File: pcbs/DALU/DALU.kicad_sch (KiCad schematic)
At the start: 1 part, among them J101 Conn_02x20_Odd_Even

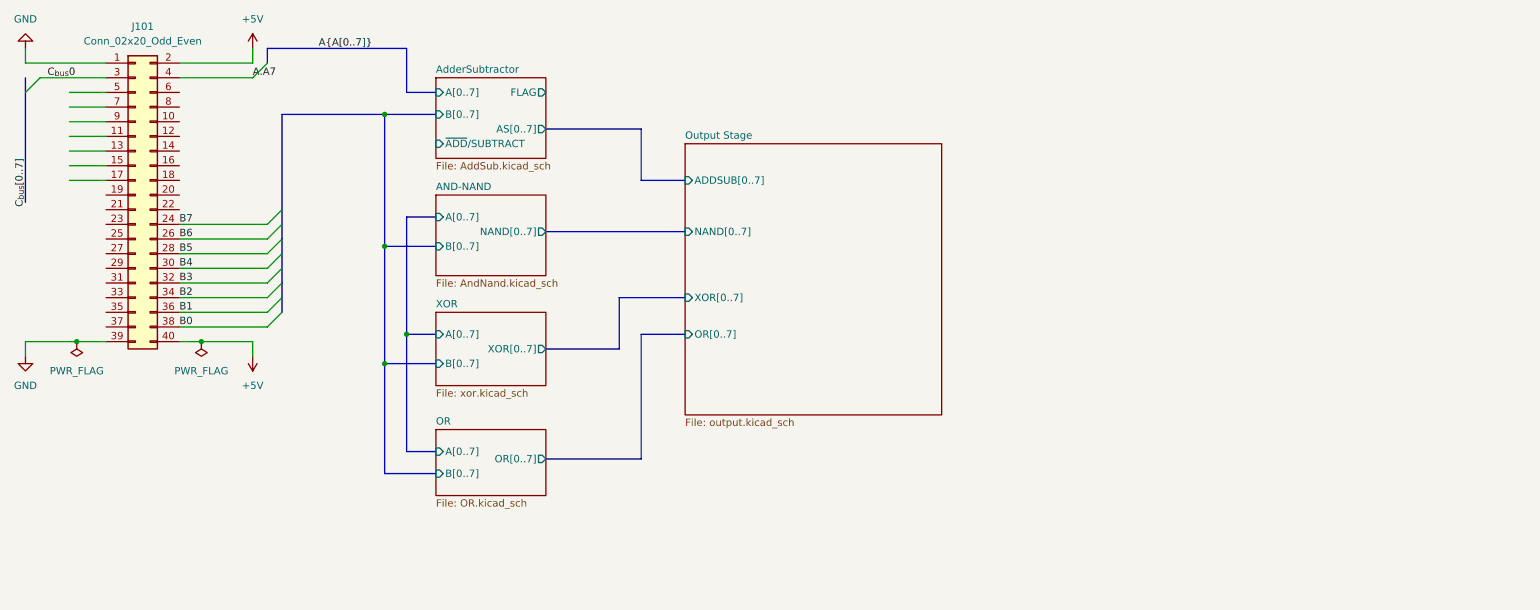
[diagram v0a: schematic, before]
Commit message: Thinking about SMD assembly. Will be rethinking
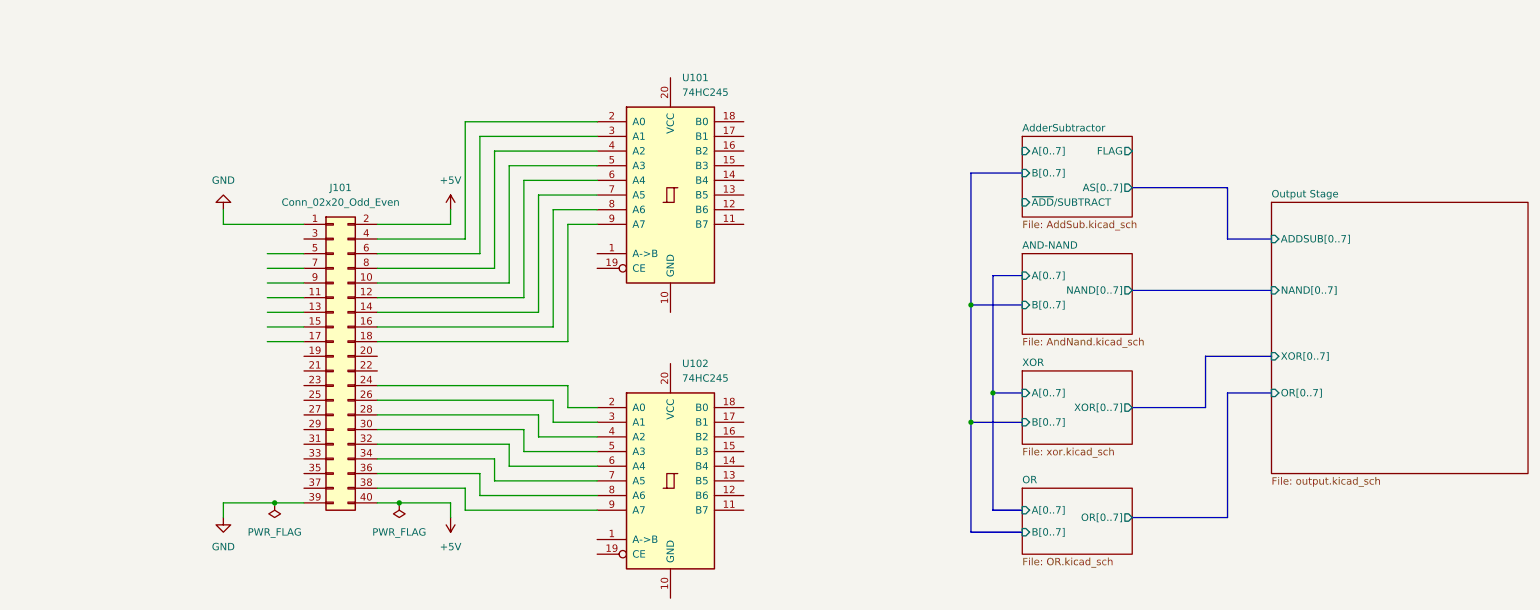
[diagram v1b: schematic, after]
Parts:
- added U101, U102: 74HC245, Package_SO:SOIC-20W_7.5x12.8mm_P1.27mm, symbol 74xx:74HC245
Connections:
- net at J101.10 (Pin_10): now also U101.5 (A3)
- net at J101.12 (Pin_12): now also U101.6 (A4)
- net at J101.14 (Pin_14): now also U101.7 (A5)
- net at J101.16 (Pin_16): now also U101.8 (A6)
- net at J101.18 (Pin_18): now also U101.9 (A7)
- net at J101.6 (Pin_6): now also U101.3 (A1)
- net at J101.8 (Pin_8): now also U101.4 (A2)
- net A.A7: no longer names the net of J101.4 (Pin_4)
- net A.A7: now also U101.2 (A0)
- net B0: no longer names the net of J101.38 (Pin_38)
- net B0: now also U102.9 (A7)
- net B1: no longer names the net of J101.36 (Pin_36)
- net B1: now also U102.8 (A6)
- net B2: no longer names the net of J101.34 (Pin_34)
- net B2: now also U102.7 (A5)
- net B3: no longer names the net of J101.32 (Pin_32)
- net B3: now also U102.6 (A4)
- net B4: no longer names the net of J101.30 (Pin_30)
- net B4: now also U102.5 (A3)
- net B5: no longer names the net of J101.28 (Pin_28)
- net B5: now also U102.4 (A2)
- net B6: no longer names the net of J101.26 (Pin_26)
- net B6: now also U102.3 (A1)
- net B7: no longer names the net of J101.24 (Pin_24)
- net B7: now also U102.2 (A0)
- net C_{bus}0: no longer names the net of J101.3 (Pin_3)
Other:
- moved on the sheet: J101
